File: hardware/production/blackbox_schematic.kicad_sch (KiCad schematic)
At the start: 0 parts

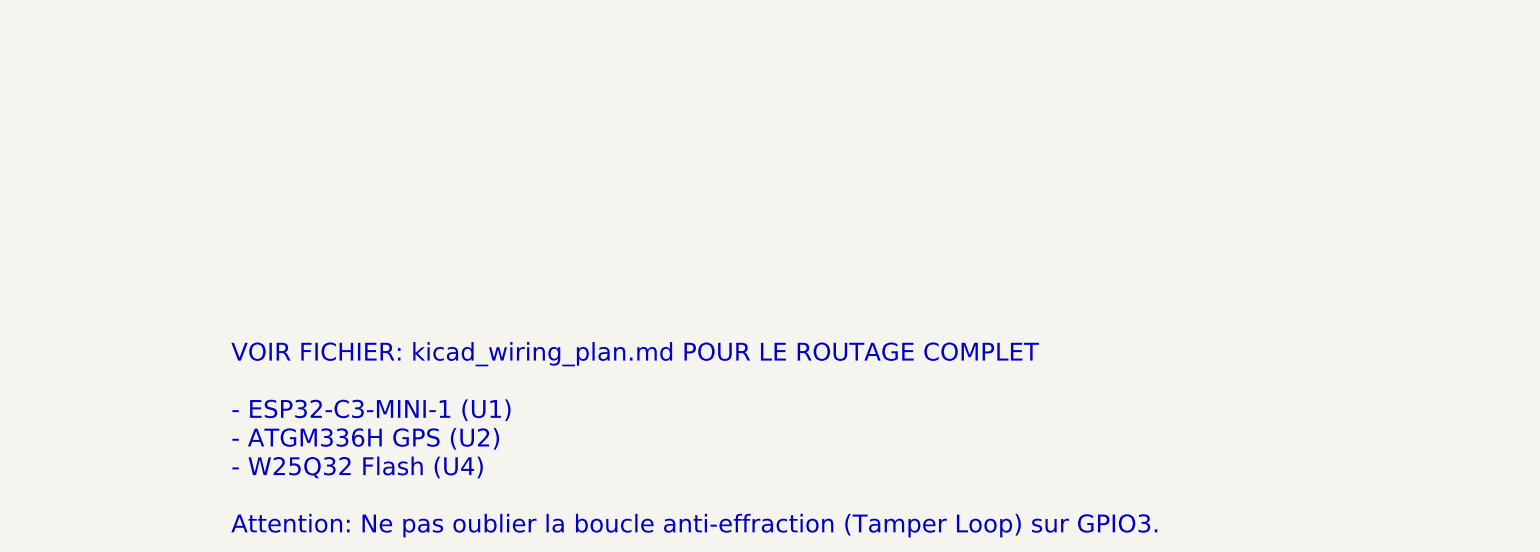
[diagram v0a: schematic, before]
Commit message: chore: save current work and push
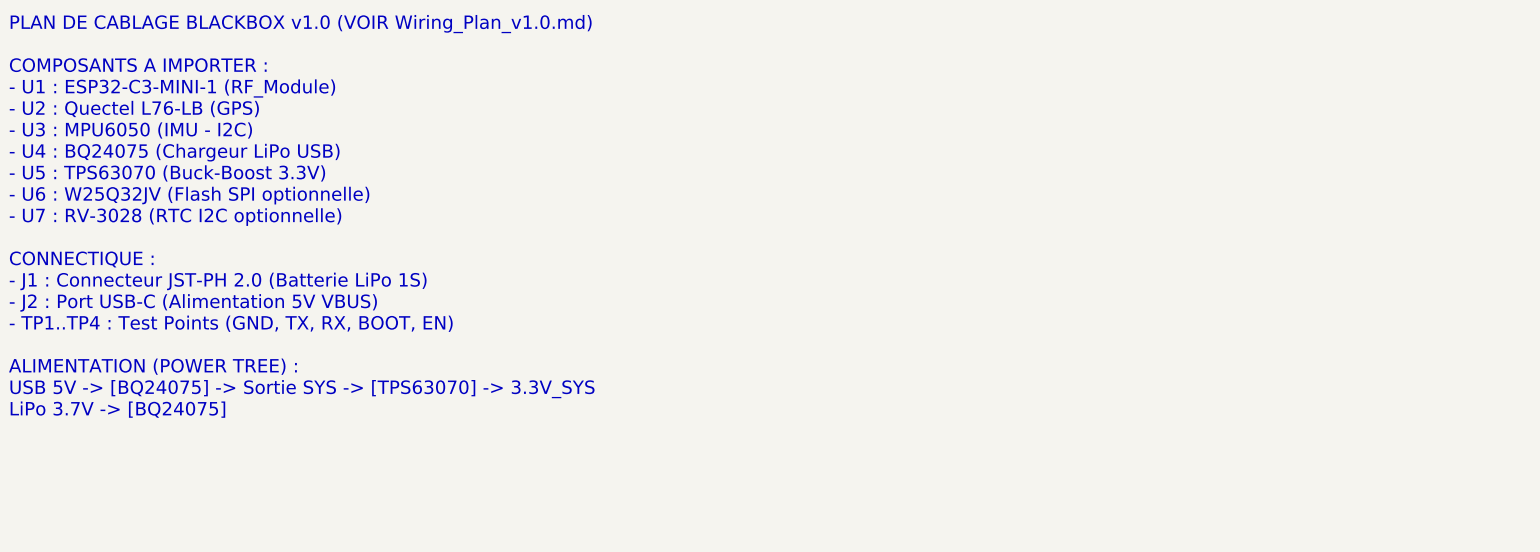
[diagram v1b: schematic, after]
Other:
- note added: "PLAN DE CABLAGE BLACKBOX v1.0 (VOIR Wiring_Plan_v1.0.md) COMPOSANTS A IMPORTER : - U1 : ESP32-C3-MINI-1 (RF_Module) - U2 : Quectel L76-LB (GPS) - U3 : MPU6050 (IMU - I2C) - U4 : BQ24075 (Chargeur LiPo USB) - U5 : TPS63070 (Buck-Boost 3.3V) - U6 : W25Q32JV (Flash SPI optionnelle) - U7 : RV-3028 (RTC I2C optionnelle) CONNECTIQUE : - J1 : Connecteur JST-PH 2.0 (Batterie LiPo 1S) - J2 : Port USB-C (A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"
- note removed: "VOIR FICHIER: kicad_wiring_plan.md POUR LE ROUTAGE COMPLET - ESP32-C3-MINI-1 (U1) - ATGM336H GPS (U2) - W25Q32 Flash (U4) Attention: Ne pas oublier la boucle anti-effraction (Tamper Loop) sur GPIO3."
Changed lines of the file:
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@@
     (company "mon50ccetmoi")
   )
-  (text "VOIR FICHIER: kicad_wiring_plan.md POUR LE ROUTAGE COMPLET\n\n- ESP32-C3-MINI-1 (U1)\n- ATGM336H GPS (U2)\n- W25Q32 Flash (U4)\n\nAttention: Ne pas oublier la boucle anti-effraction (Tamper Loop) sur GPIO3." (at 100 100 0)
-    (effects (font (size 4 4) (thickness 0.6)) (justify left))
+  (text "PLAN DE CABLAGE BLACKBOX v1.0 (VOIR Wiring_Plan_v1.0.md)\n\nCOMPOSANTS A IMPORTER :\n- U1 : ESP32-C3-MINI-1 (RF_Module)\n- U2 : Quectel L76-LB (GPS)\n- U3 : MPU6050 (IMU - I2C)\n- U4 : BQ24075 (Chargeur LiPo USB)\n- U5 : TPS63070 (Buck-Boost 3.3V)\n- U6 : W25Q32JV (Flash SPI optionnelle)\n- U7 : RV-3028 (RTC I2C optionnelle)\n\nCONNECTIQUE :\n- J1 : Connecteur JST-PH 2.0 (Batterie LiPo 1S)\n- J2 : Port USB-C (Alimentation 5V VBUS)\n- TP1..TP4 : Test Points (GND, TX, RX, BOOT, EN)\n\nALIMENTATION (POWER TREE) :\nUSB 5V -> [BQ24075] -> Sortie SYS -> [TPS63070] -> 3.3V_SYS\nLiPo 3.7V -> [BQ24075]" (at 50 50 0)
+    (effects (font (size 3 3) (thickness 0.4)) (justify left))
   )
 )
